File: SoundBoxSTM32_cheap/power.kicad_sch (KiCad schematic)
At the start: 22 parts, among them Q2 FS8205A, Q3 AO3401A, SW1 OS102011MA1QN1, U3 1043, U4 DW01A, U5 TPS3840DL35DBVR, U6 TLV75733PDBVR

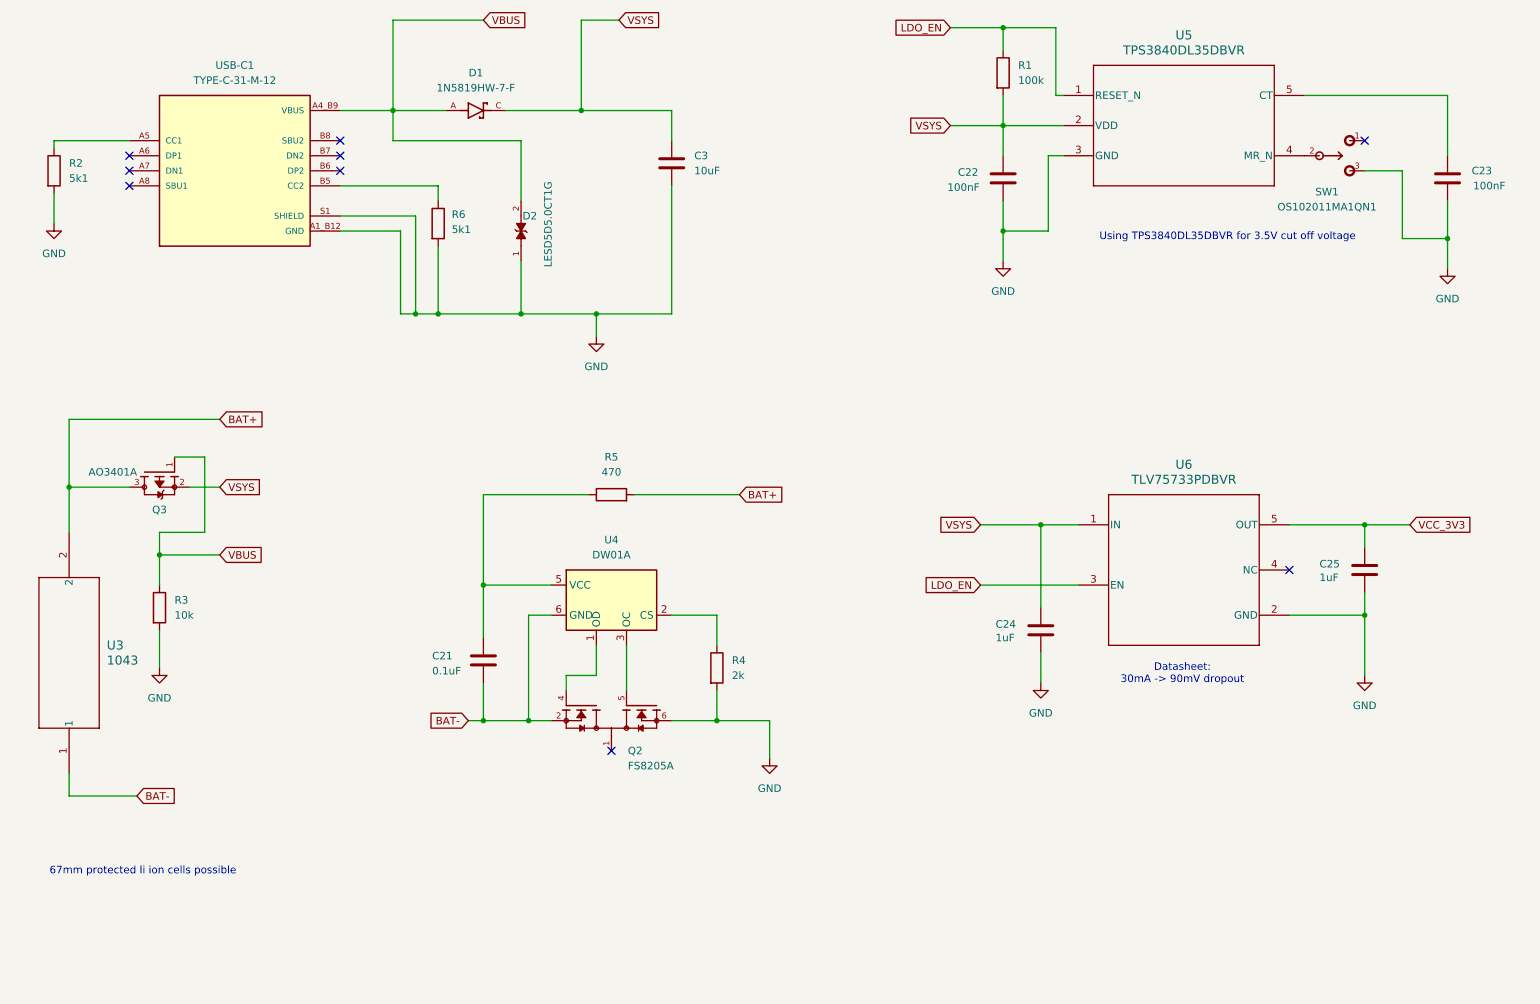
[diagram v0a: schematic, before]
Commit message: Finished LoveBox, Finished Rubberducky
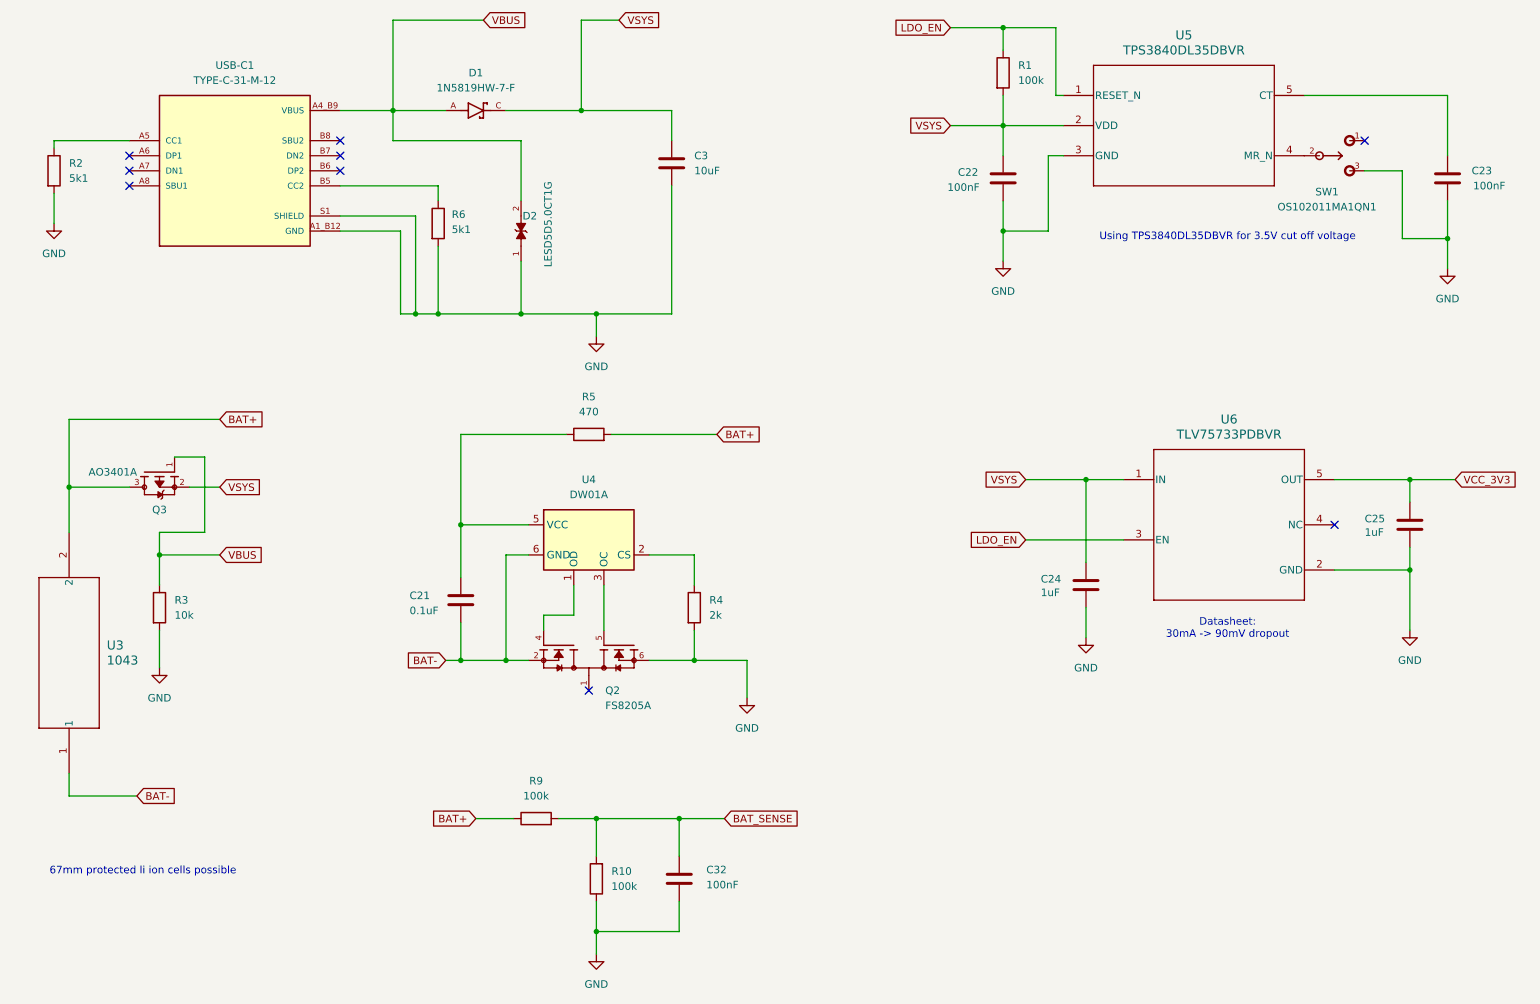
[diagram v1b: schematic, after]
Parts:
- added C32: 100nF, Capacitor_SMD:C_0603_1608Metric, symbol Device:C
- added R10, R9: 100k, Resistor_SMD:R_0603_1608Metric, symbol Device:R
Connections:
- net BAT+: now also R9.1
- net GND: now also C32.2, R10.1
- new net BAT_SENSE: C32.1, R10.2, R9.2
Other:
- moved on the sheet: C21, C24, C25, Q2, R4, R5, U4, U6
